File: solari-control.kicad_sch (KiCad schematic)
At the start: 84 parts, among them J1 Conn_01x05, J2 AVR-ISP-6, J3 Conn_01x04, J4 DIL8, J5 Conn_01x04, J6 Conn_01x05, Q1 AO3401A, Q2 AO3401A, Q3 AO3400A, Q4 AO3400A, Q5 BC327, Q6 BC327, U1 VO0631T, U2 ATmega328P-A, U3 VO0631T, U4 VO0631T, U5 VO0631T, U6 VO0631T, U7 VO0631T, U8 VO0631T, Y1 14.7456 MHz

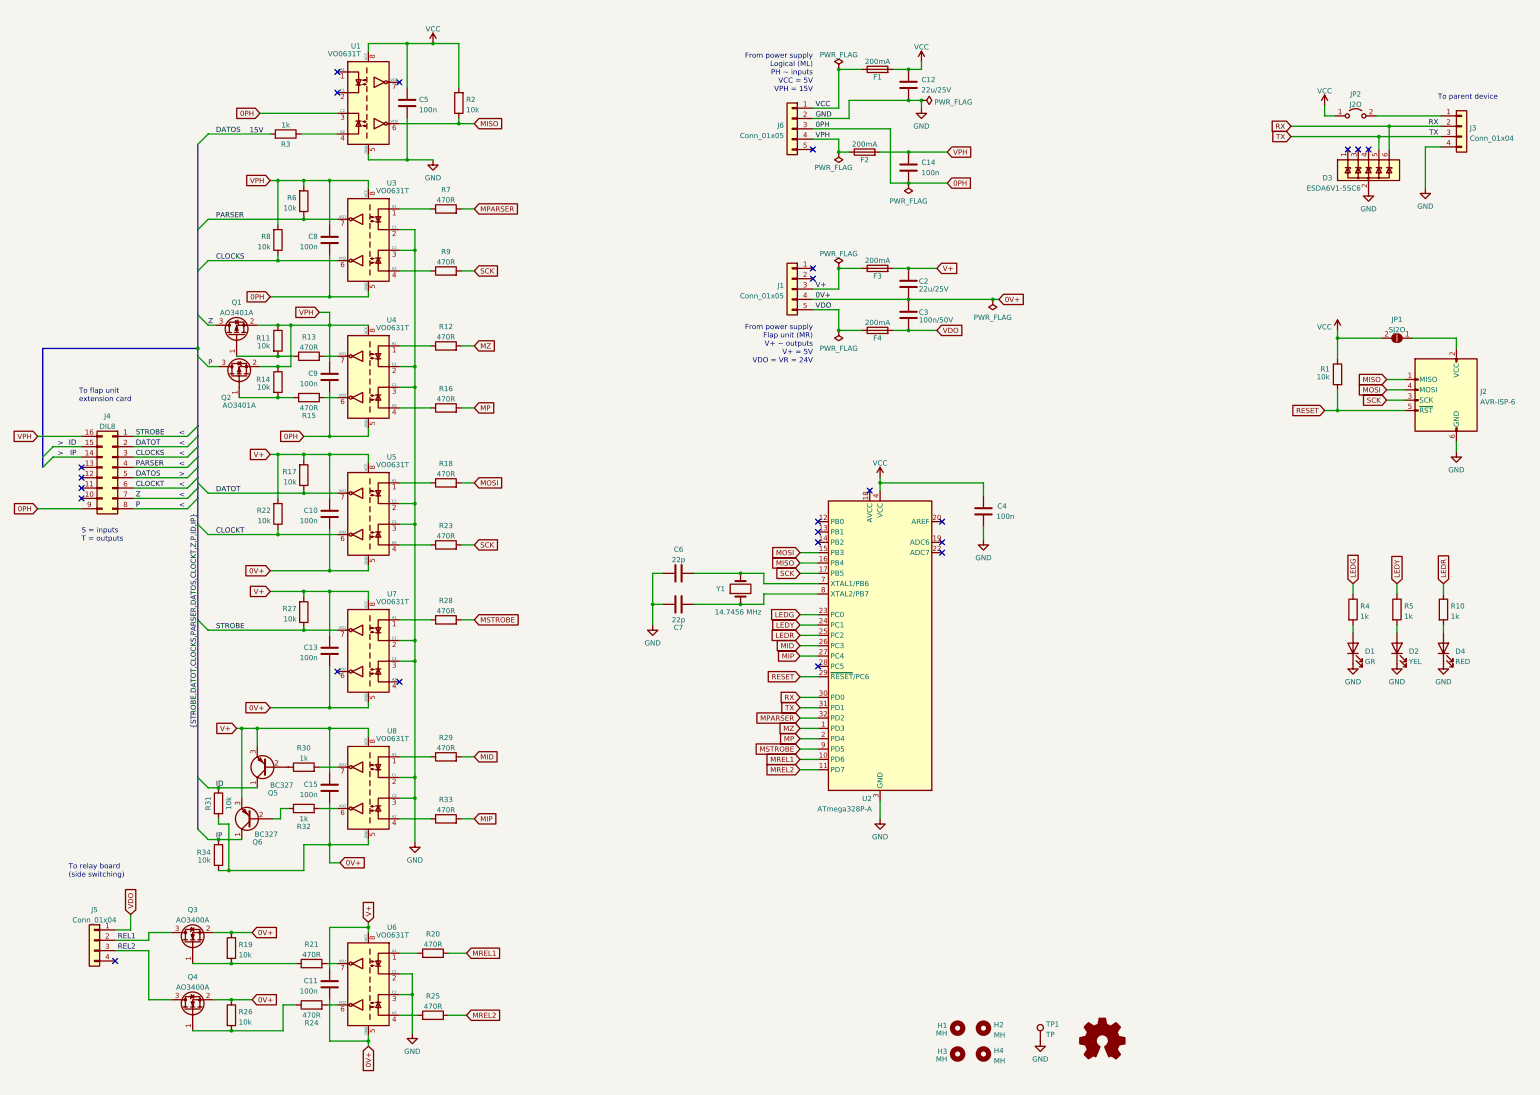
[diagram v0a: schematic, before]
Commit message: Add transistors for 15V outputs.
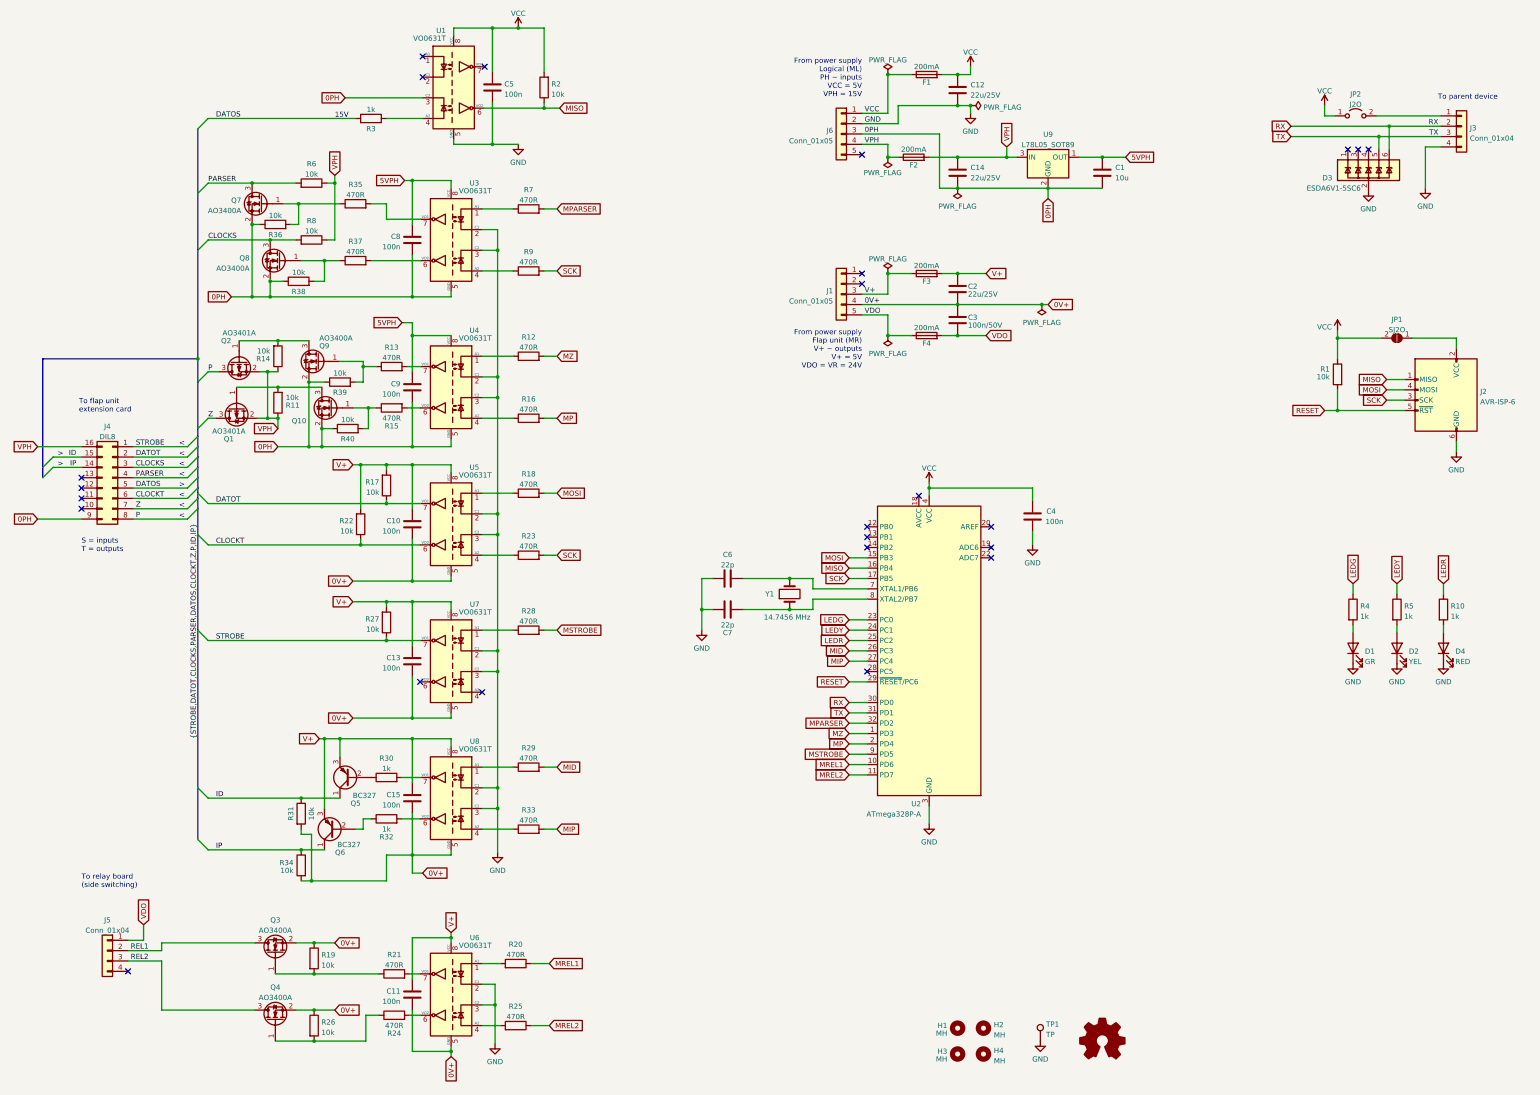
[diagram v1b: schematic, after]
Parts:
- added C1: 10u, symbol Device:C
- added Q10, Q7, Q8, Q9: AO3400A, Package_TO_SOT_SMD:SOT-23, symbol Transistor_FET:AO3400A
- added R35, R37: 470R, symbol Device:R
- added R36, R38, R39, R40: 10k, symbol Device:R
- added U9: L78L05_SOT89, Package_TO_SOT_SMD:SOT-89-3, symbol Regulator_Linear:L78L05_SOT89
- C14: value 100n -> 22u/25V
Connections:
- net 0PH: now also C1.2, Q10.2 (S), Q7.2 (S), Q8.2 (S), Q9.2 (S), R36.1, R38.1, R39.1, R40.1, U9.2 (GND)
- net CLOCKS: now also R8.2, Q8.3 (D); no longer R8.1, U3.6 (VO2)
- net PARSER: now also R6.2, Q7.3 (D); no longer R6.1, U3.7 (VO1)
- net VPH: now also R6.1, R8.1, U9.3 (IN); no longer C8.1, C9.1, R6.2, R8.2, U3.8 (VCC), U4.8 (VCC)
- net at Q1.1 (G), R11.2: now also Q10.3 (D); no longer R13.1
- net at Q2.1 (G), R14.2: now also Q9.3 (D); no longer R15.1
- new net: Q10.1 (G), R15.1, R40.2
- new net: Q7.1 (G), R35.1, R36.2
- new net: R35.2, U3.7 (VO1)
- new net: R37.2, U3.6 (VO2)
- new net: Q9.1 (G), R13.1, R39.2
- new net: Q8.1 (G), R37.1, R38.2
- new net 5VPH: C1.1, C8.1, C9.1, U3.8 (VCC), U4.8 (VCC), U9.1 (OUT)
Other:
- moved on the sheet: C10, C11, C12, C13, C14, C15, C2, C3, C4, C5, C6, C7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
